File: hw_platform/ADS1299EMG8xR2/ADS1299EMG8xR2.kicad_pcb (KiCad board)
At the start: 2 copper layers, 81 parts, among them U1 PJ-325-5P, U10 LM1117-5.0, U11 LM1117-3.3, U12 LM1117-5.0, U13 ESP32-DevKitC, U2 PJ-325-5P, U3 PJ-325-5P, U4 PJ-325-5P, U5 PJ-325-5P, U6 PJ-325-5P, U7 PJ-325-5P, U8 PJ-325-5P, U9 ADS1299

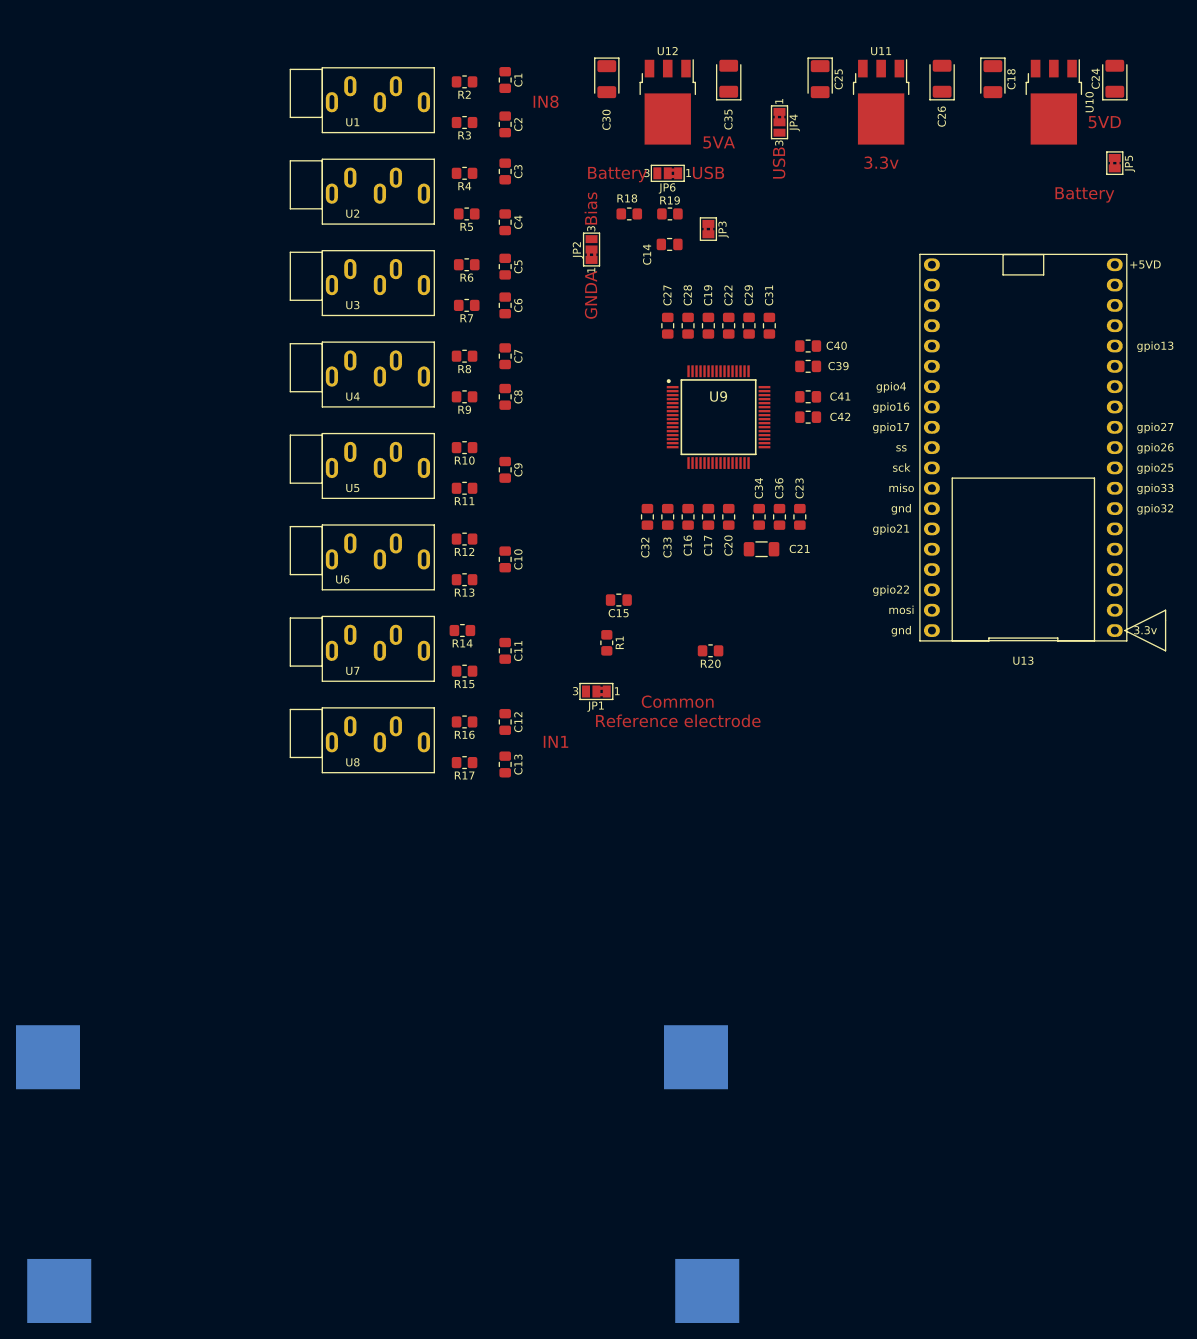
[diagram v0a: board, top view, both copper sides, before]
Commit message: partial routed
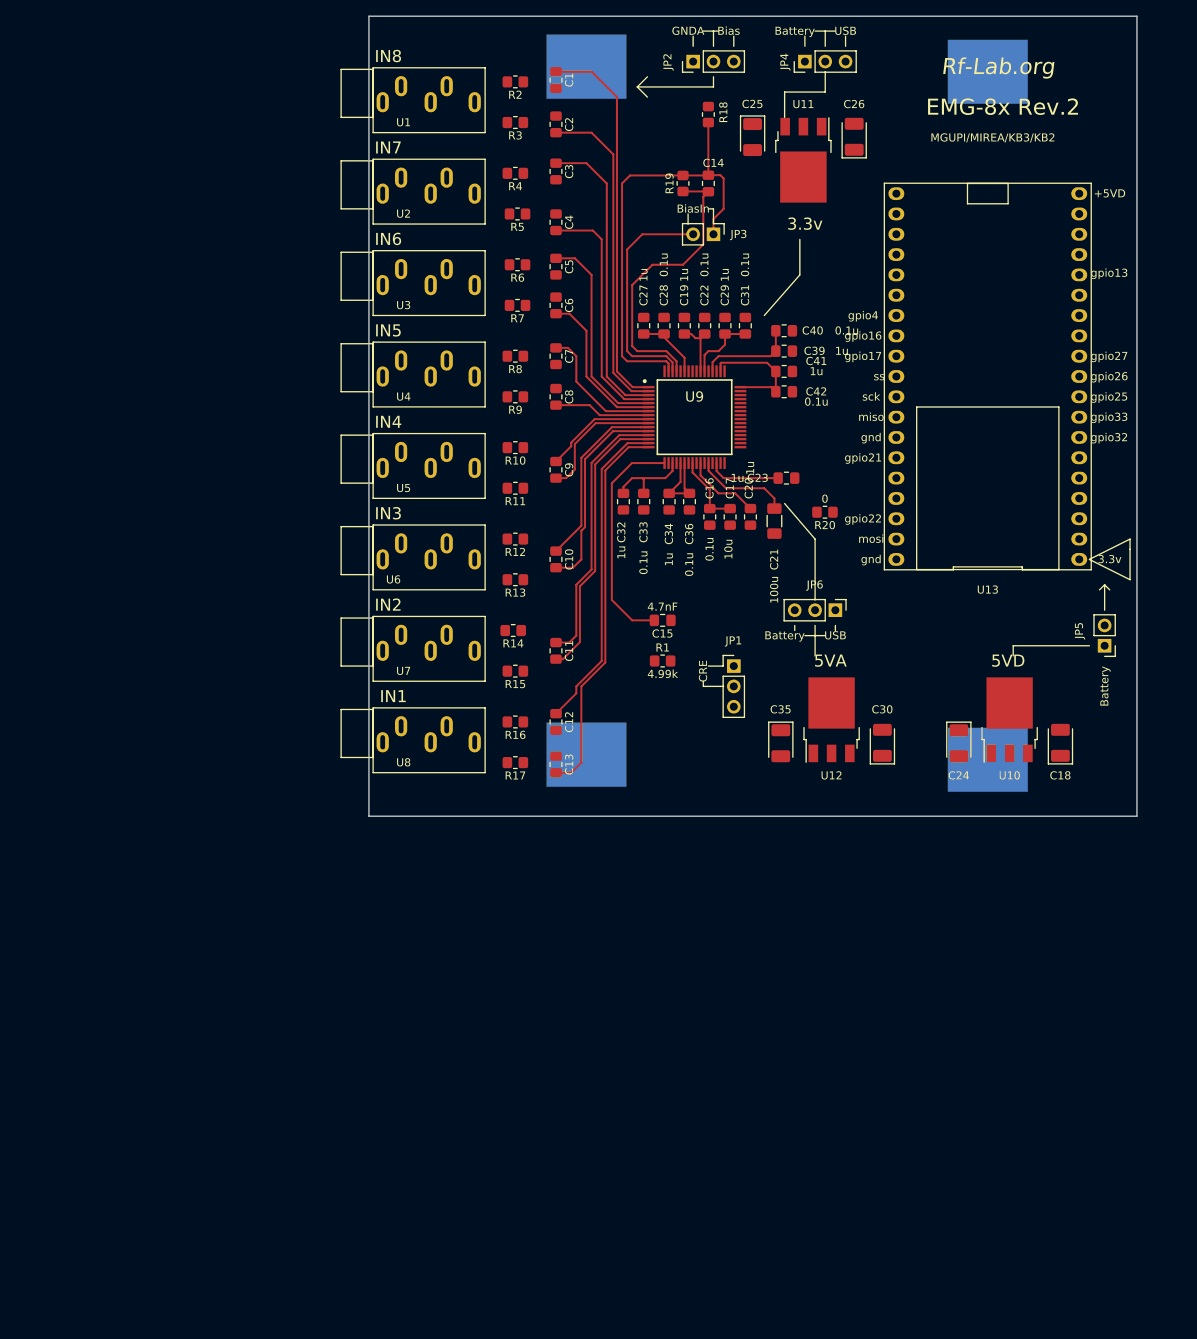
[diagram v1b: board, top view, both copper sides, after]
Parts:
- JP1, JP2, JP4, JP6: footprint Jumper:SolderJumper-3_P1.3mm_Bridged2Bar12_Pad1.0x1.5mm_NumberLabels -> Connector_PinHeader_2.54mm:PinHeader_1x03_P2.54mm_Vertical
- JP3, JP5: footprint Jumper:SolderJumper-2_P1.3mm_Bridged2Bar_Pad1.0x1.5mm -> Connector_PinHeader_2.54mm:PinHeader_1x02_P2.54mm_Vertical
- moved BT1 133.0 mm to (173.4, 70.9), turned to 270 degrees
- moved C30 89.8 mm to (160.2, 111.8), turned to 90 degrees
- moved C24 85.3 mm to (169.7, 111.9), turned to 270 degrees
- moved BT2 85.2 mm to (123.2, 70.3), turned to 90 degrees
- moved C18 83.4 mm to (182.4, 111.8), turned to 90 degrees
- moved C35 83.3 mm to (147.5, 111.9), turned to 270 degrees
- moved U12 79.9 mm to (153.8, 109.0), turned to 90 degrees
- moved U10 77.4 mm to (176.1, 109.0), turned to 90 degrees
- moved JP5 60.3 mm to (188.0, 99.7), turned to 180 degrees
- moved JP6 58.5 mm to (154.3, 95.2), turned to 270 degrees
- moved JP2 26.7 mm to (136.5, 26.7)
- moved R20 22.5 mm to (153.0, 83.0)
- moved JP1 17.5 mm to (141.6, 102.2), turned to 0 degrees
- moved R18 15.9 mm to (138.4, 33.3), turned to 90 degrees
- moved C26 13.2 mm to (156.7, 36.1)
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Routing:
- net Net-(C14-Pad2): track 0.00 -> 56.1 mm
- net Net-(C13-Pad2): track 0.00 -> 48.1 mm
- net Net-(C1-Pad1): track 0.00 -> 48.0 mm
- net Net-(C2-Pad2): track 0.00 -> 41.0 mm
- net Net-(C12-Pad1): track 0.00 -> 40.2 mm
- net +5VA: track 0.00 -> 39.0 mm
- net Net-(C3-Pad1): track 0.00 -> 37.7 mm
- net Net-(C14-Pad1): track 0.00 -> 36.2 mm
- net Net-(C11-Pad2): track 0.00 -> 34.9 mm
- net Net-(C11-Pad1): track 0.00 -> 33.9 mm
- net Net-(C4-Pad2): track 0.00 -> 30.4 mm
- net Net-(JP3-Pad2): track 0.00 -> 29.1 mm
- net Net-(C15-Pad2): track 0.00 -> 28.6 mm
- net +3V3: track 0.00 -> 27.7 mm
- net Net-(C5-Pad1): track 0.00 -> 26.5 mm
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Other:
- board outline added: 96 x 100 mm
- board text added: "BiasIn"
- board text added: "CRE"
- board text added: "EMG-8x Rev.2"
- board text added: "IN2"
- board text added: "IN3"
- board text added: "IN4"
- board text added: "IN5"
- board text added: "IN6"
- board text added: "IN7"
- board text added: "MGUPI/MIREA/KB3/KB2"
- board text added: "Rf-Lab.org"
- board text removed: "Common Reference electrode"
